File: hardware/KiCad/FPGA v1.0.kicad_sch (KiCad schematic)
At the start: 4 parts

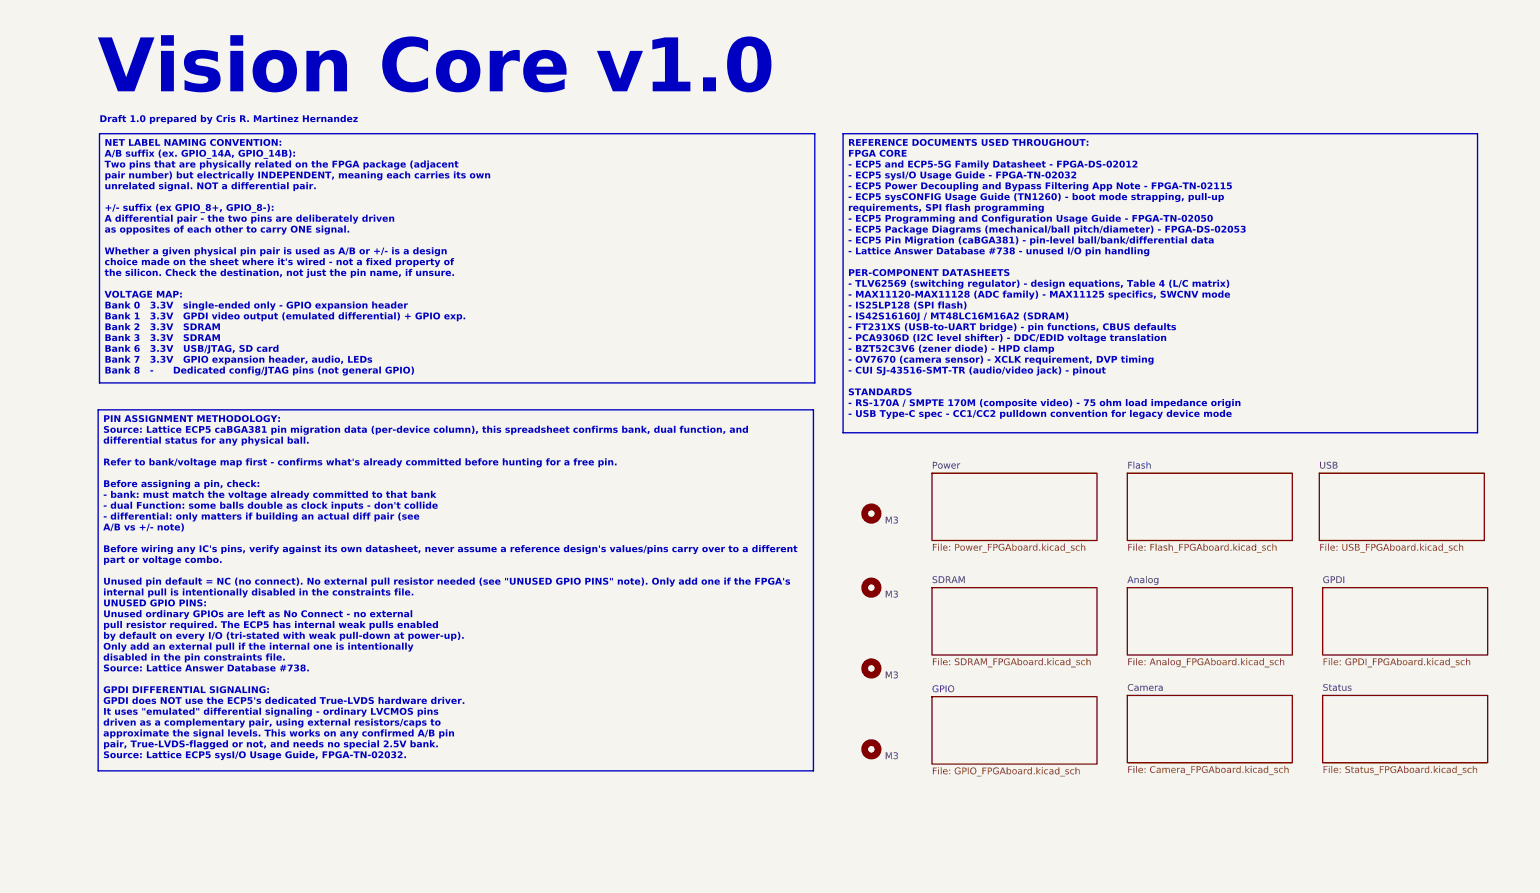
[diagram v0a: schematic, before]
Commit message: Add files via upload
v1.1
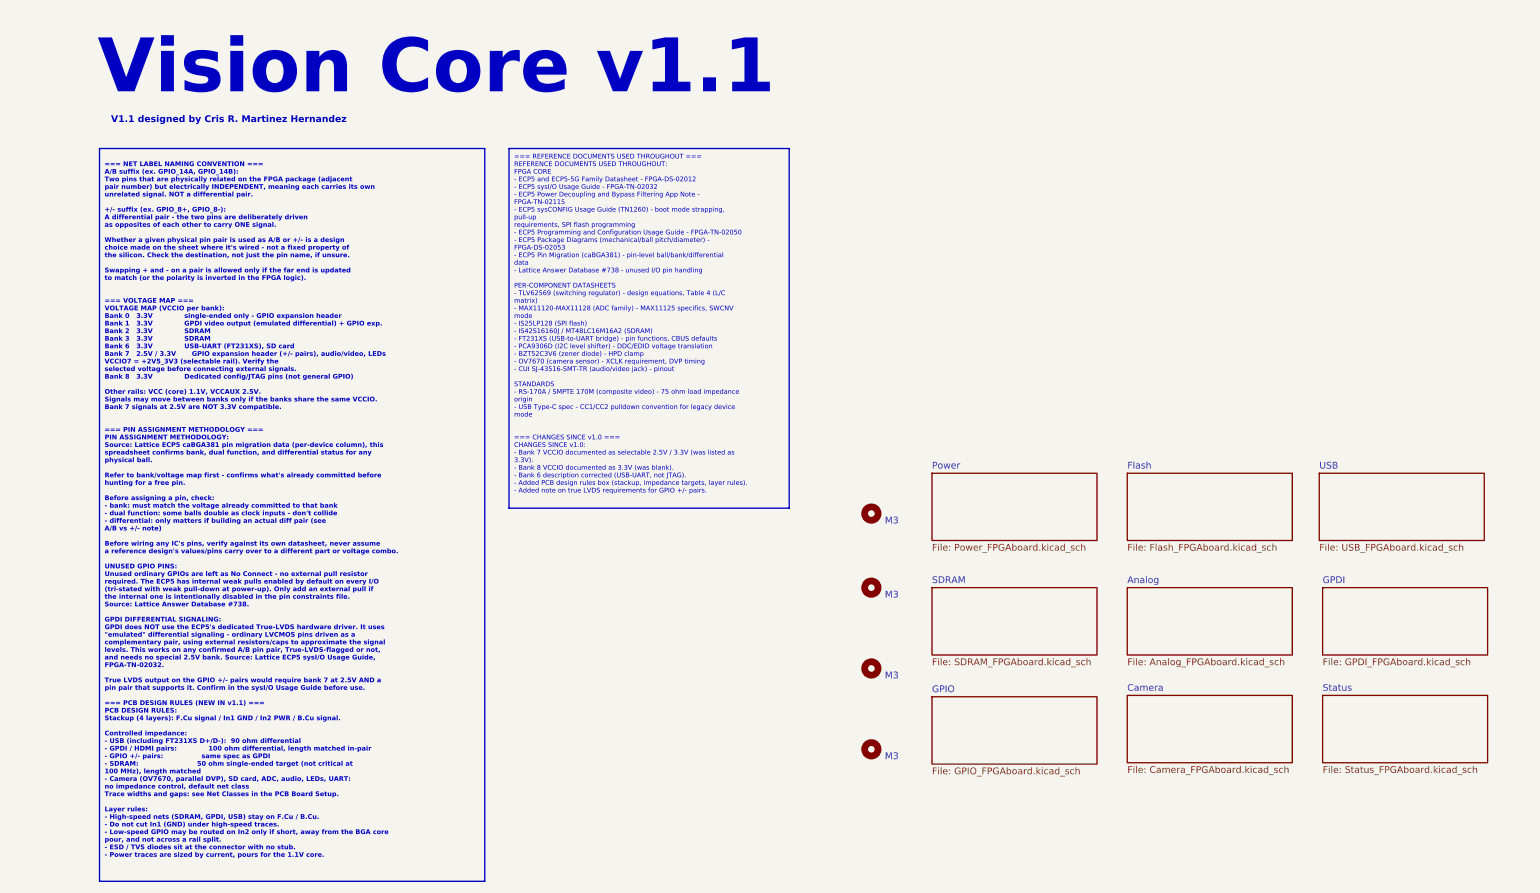
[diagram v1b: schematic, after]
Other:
- note added: "V1.1 designed by Cris R. Martinez Hernandez"
- note added: "Vision Core v1.1"
- note removed: "Draft 1.0 prepared by Cris R. Martinez Hernandez"
- note removed: "Vision Core v1.0"
